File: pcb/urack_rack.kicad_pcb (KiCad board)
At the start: 2 copper layers, 250 x 250 mm, 11 parts, among them J1 Conn_01x40, J2 Conn_01x40, J3 Conn_01x40, J4 Conn_01x40, J5 Conn_01x40, J6 Conn_01x40, J7 Conn_01x40, J8 Conn_01x40, J9 Conn_01x40

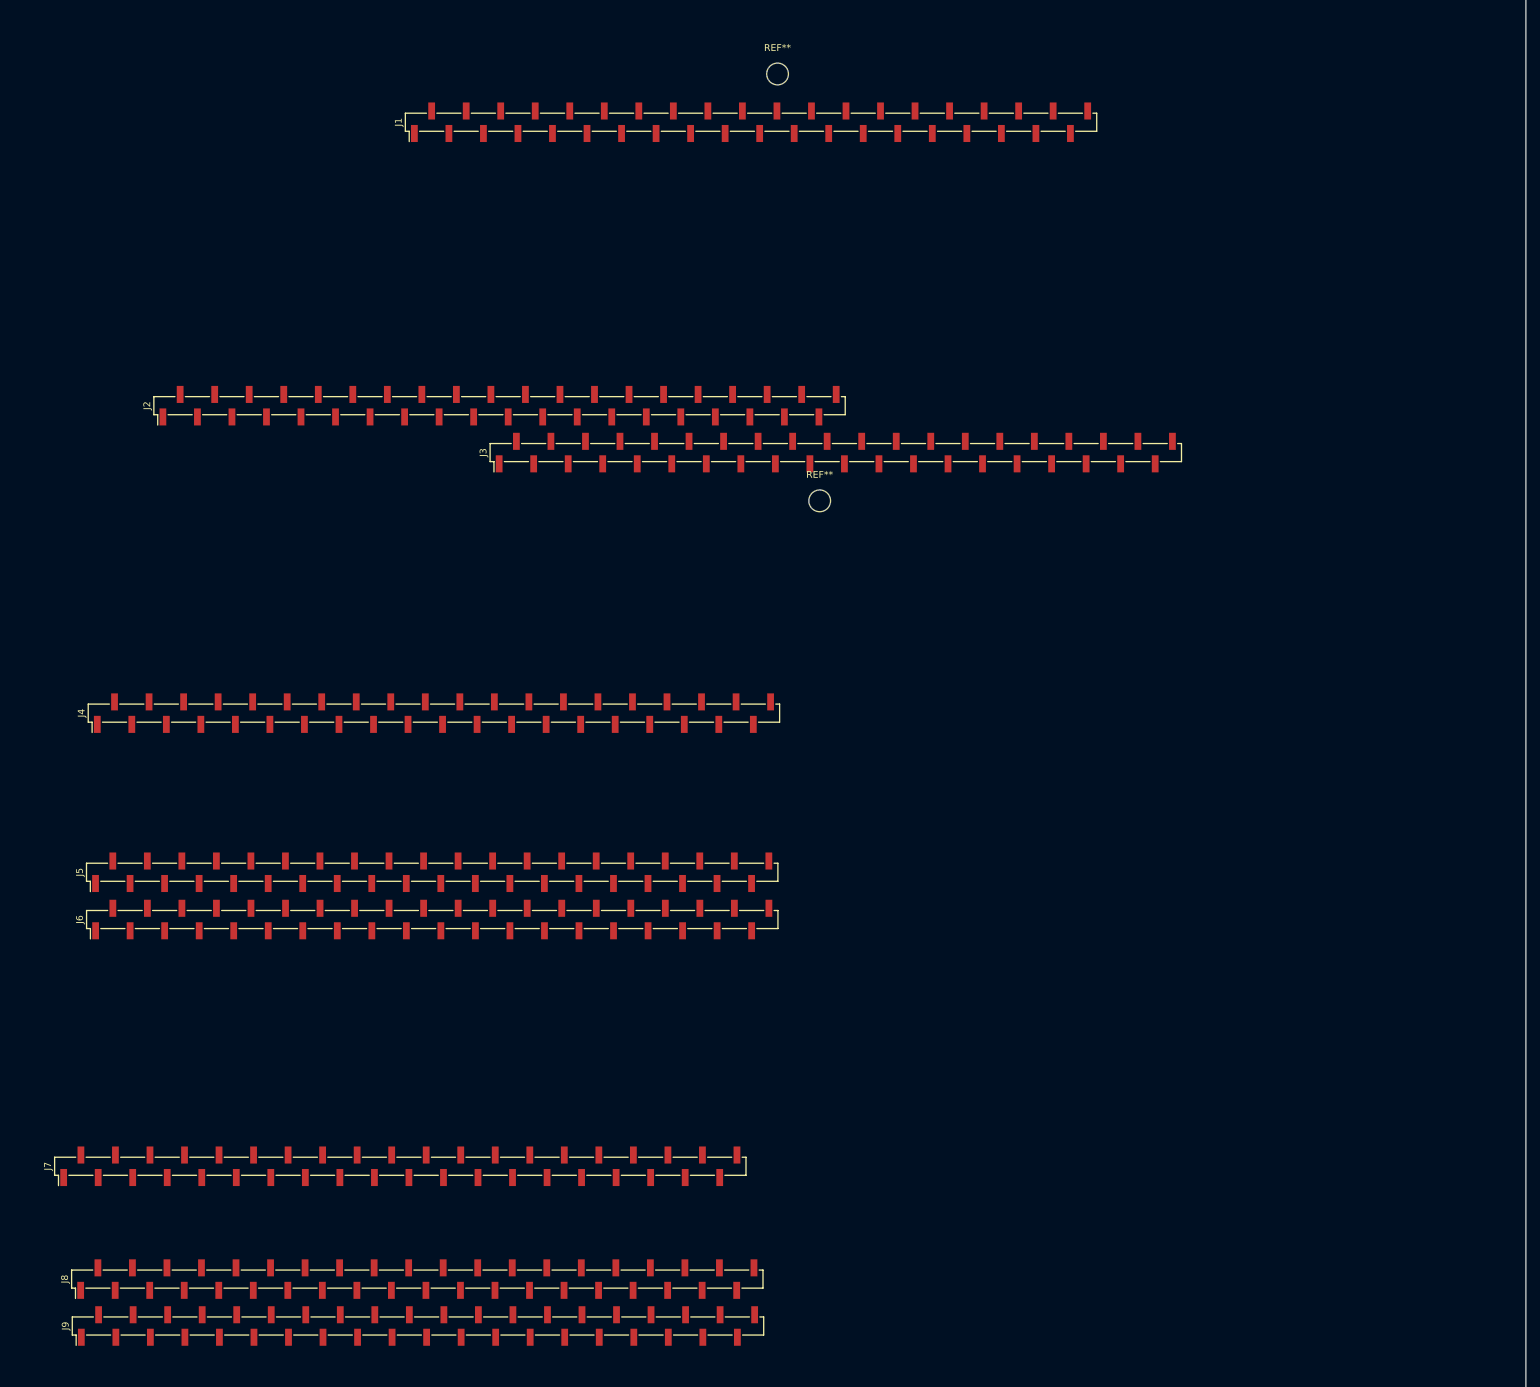
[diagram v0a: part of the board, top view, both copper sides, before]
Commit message: update pcb
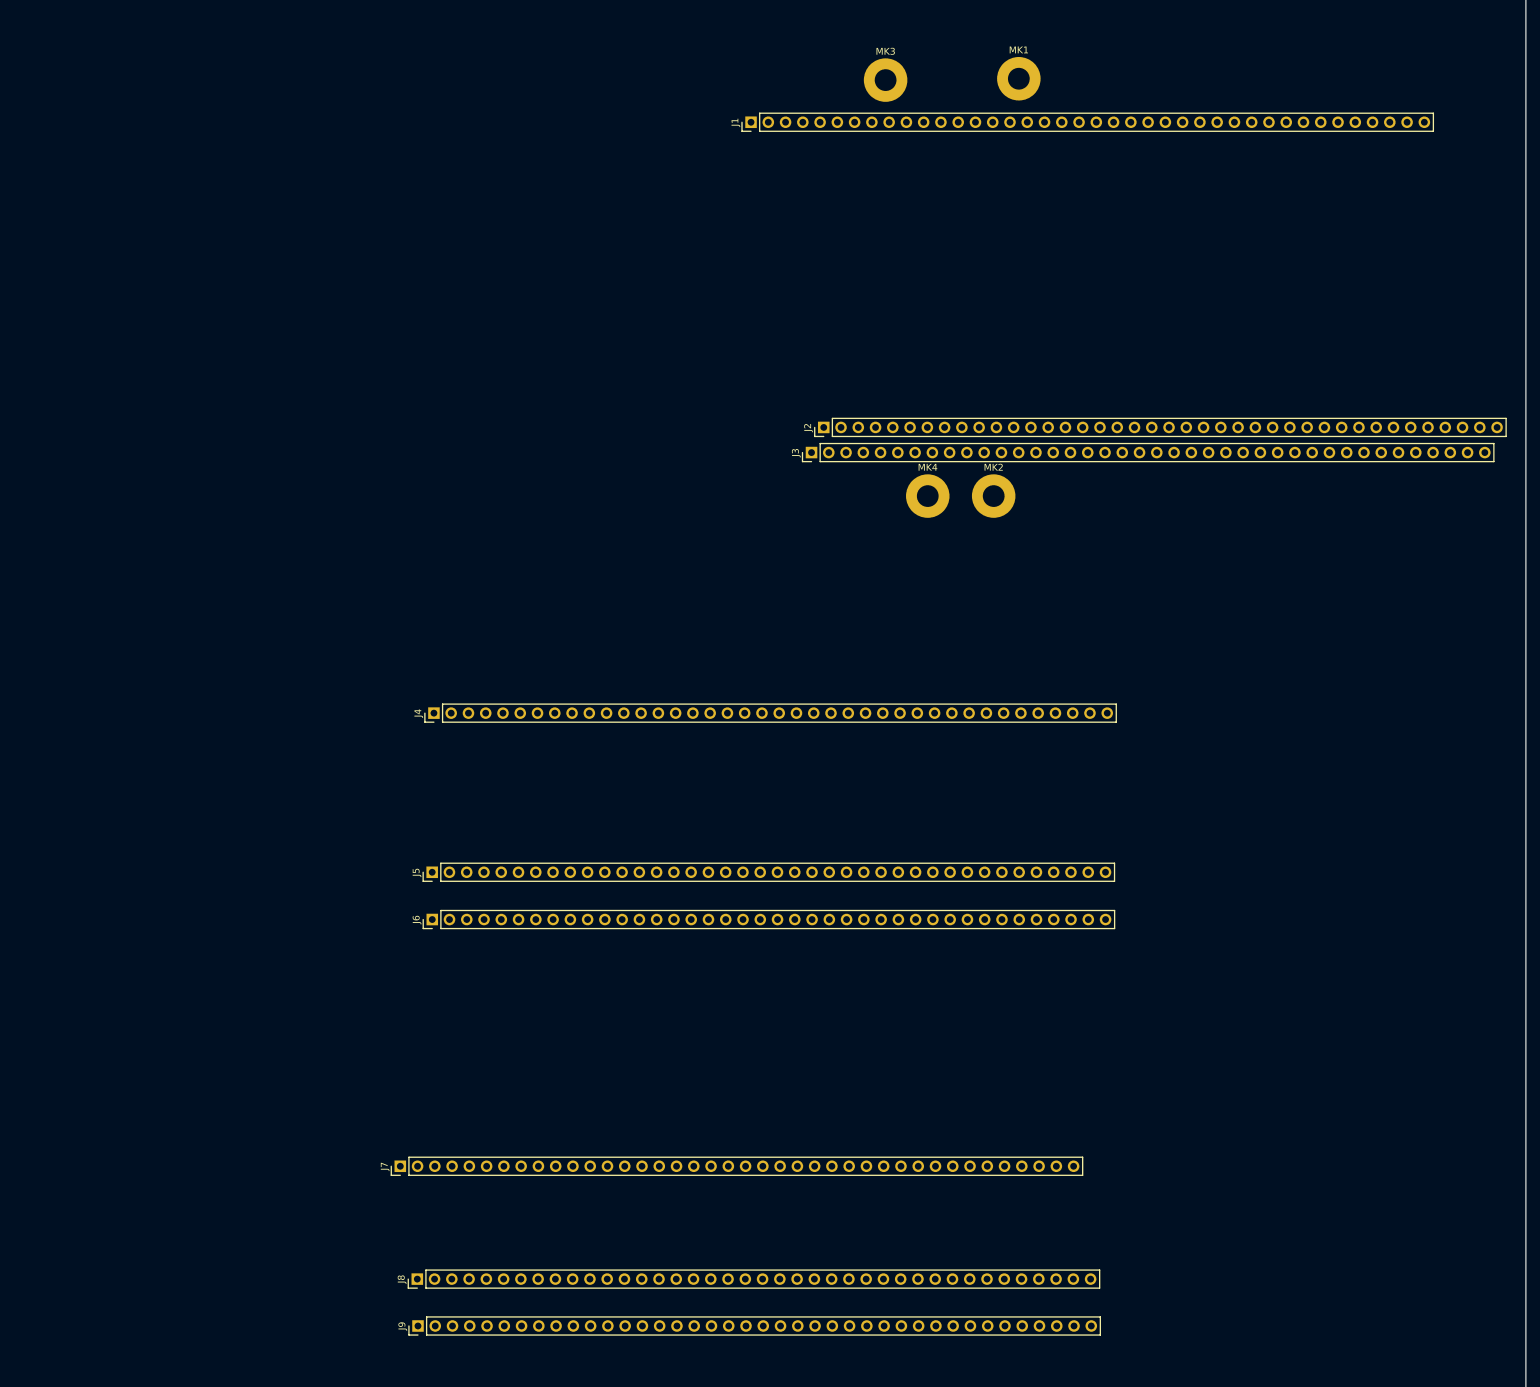
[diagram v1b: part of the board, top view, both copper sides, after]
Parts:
- removed REF** (x2): MountingHole_3.2mm_M3_ISO7380, Mounting_Holes:MountingHole_3.2mm_M3_ISO7380
- added MK1: Mounting_Hole, Mounting_Holes:MountingHole_3.2mm_M3_Pad, F.Cu at (195.4, 62.2)
- added MK2: Mounting_Hole, Mounting_Holes:MountingHole_3.2mm_M3_Pad, F.Cu at (191.7, 123.6)
- added MK3: Mounting_Hole, Mounting_Holes:MountingHole_3.2mm_M3_Pad, F.Cu at (175.8, 62.4)
- added MK4: Mounting_Hole, Mounting_Holes:MountingHole_3.2mm_M3_Pad, F.Cu at (182.0, 123.6)
- J1, J2, J3, J4, J5, J6, J7, J8, J9: footprint Pin_Headers:Pin_Header_Straight_1x40_Pitch2.54mm_SMD_Pin1Left -> Pin_Headers:Pin_Header_Straight_1x40_Pitch2.54mm
- moved J2 47.8 mm to (166.7, 113.5)
- moved J3 3.57 mm to (164.9, 117.2)
